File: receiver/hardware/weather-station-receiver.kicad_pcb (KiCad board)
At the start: 2 copper layers, 24.9 x 52.3 mm, 11 parts, among them J1 AntennaConnector, U1 RFM69, U2 PicoW, U3 APDS-9306-065, U4 BME280

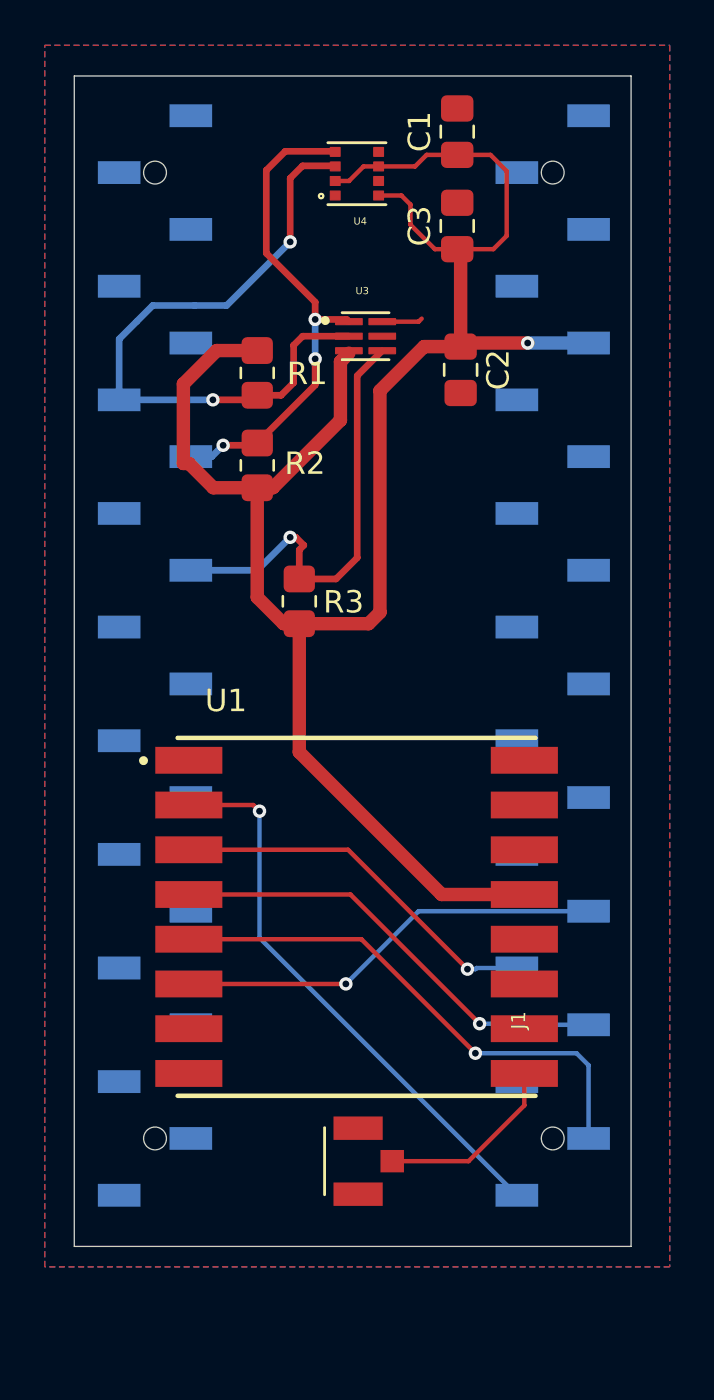
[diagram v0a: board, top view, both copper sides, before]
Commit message: Finished Layout
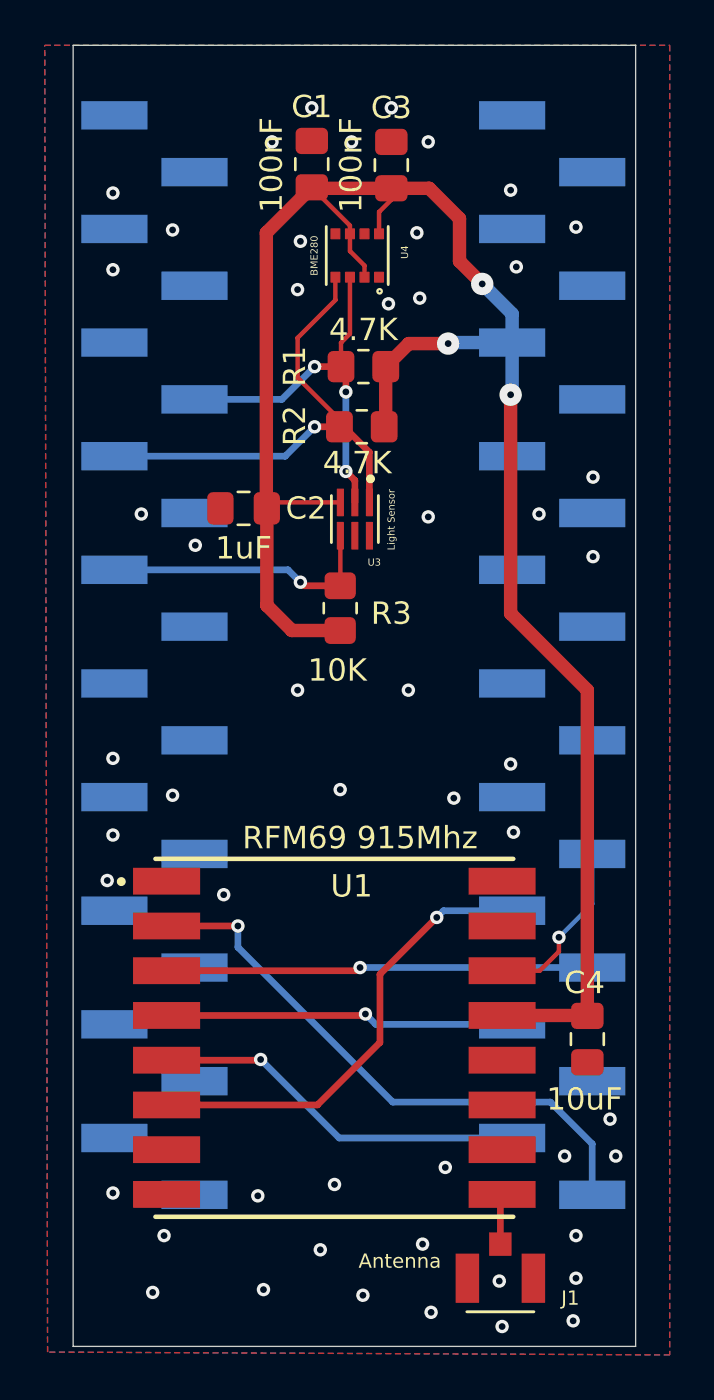
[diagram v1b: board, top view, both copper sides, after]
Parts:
- added C4: 10uF, Capacitor_SMD:C_0805_2012Metric_Pad1.18x1.45mm_HandSolder, F.Cu at (170.3, 113.0)
- J1: value AntennaConnector -> Antenna
- U1: value RFM69 -> RFM69 915Mhz
- U2: footprint Weather_Station_Receiver:Pico SMD Headers -> Weather_Station_Receiver:Pico_SMD_Headers
- U3: value APDS-9306-065 -> Light Sensor
- moved C2 11.5 mm to (154.9, 89.3), turned to 180 degrees
- moved J1 8.24 mm to (166.4, 123.7), turned to 180 degrees
- moved U3 8.19 mm to (159.9, 89.8), turned to -90 degrees
- moved C1 6.66 mm to (158.0, 73.9)
- moved U1 5.50 mm to (159.0, 113.0)
- moved R2 4.98 mm to (160.2, 85.6), turned to 180 degrees
- moved R1 4.75 mm to (160.3, 82.9), turned to 180 degrees
- moved C3 4.01 mm to (161.5, 73.9)
- moved U4 3.66 mm to (160.0, 78.0), turned to -90 degrees
- moved R3 1.85 mm to (159.3, 93.7)
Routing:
- net /I2C0_SDA: track 29.7 -> 17.6 mm, vias 2 -> 3
- net /RFM69_INTR: track 0.00 -> 7.88 mm, vias 0 -> 1
- net /APDS_INTR: track 20.1 -> 12.6 mm
- net /RFM69_CS: track 23.5 -> 17.2 mm
- net Net-(J1-SIG): track 8.37 -> 2.25 mm
- net /SPI0_CLK: track 20.3 -> 15.7 mm
- net /SPI0_MOSI: track 16.9 -> 19.1 mm
- net GND: track 1.82 -> 0.00 mm, vias 0 -> 52
- net /RFM69_RESET: track 19.2 -> 20.8 mm
- net /SPI0_MISO: track 25.2 -> 25.9 mm
- net /I2C0_SCL: track 22.4 -> 22.8 mm, vias 3 -> 1
- net +3.3V: track 92.2 -> 91.8 mm, vias 1 -> 3
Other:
- board size 24.9 x 52.3 mm -> 25.1 x 58.2 mm
